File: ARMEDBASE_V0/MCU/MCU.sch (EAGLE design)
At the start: 35 parts, among them IC1 REG1117, IC2 MEGA8-P, K1 CQ1-12V, Q1 20Mhz, Q2 2N3904, Q3 2N3904

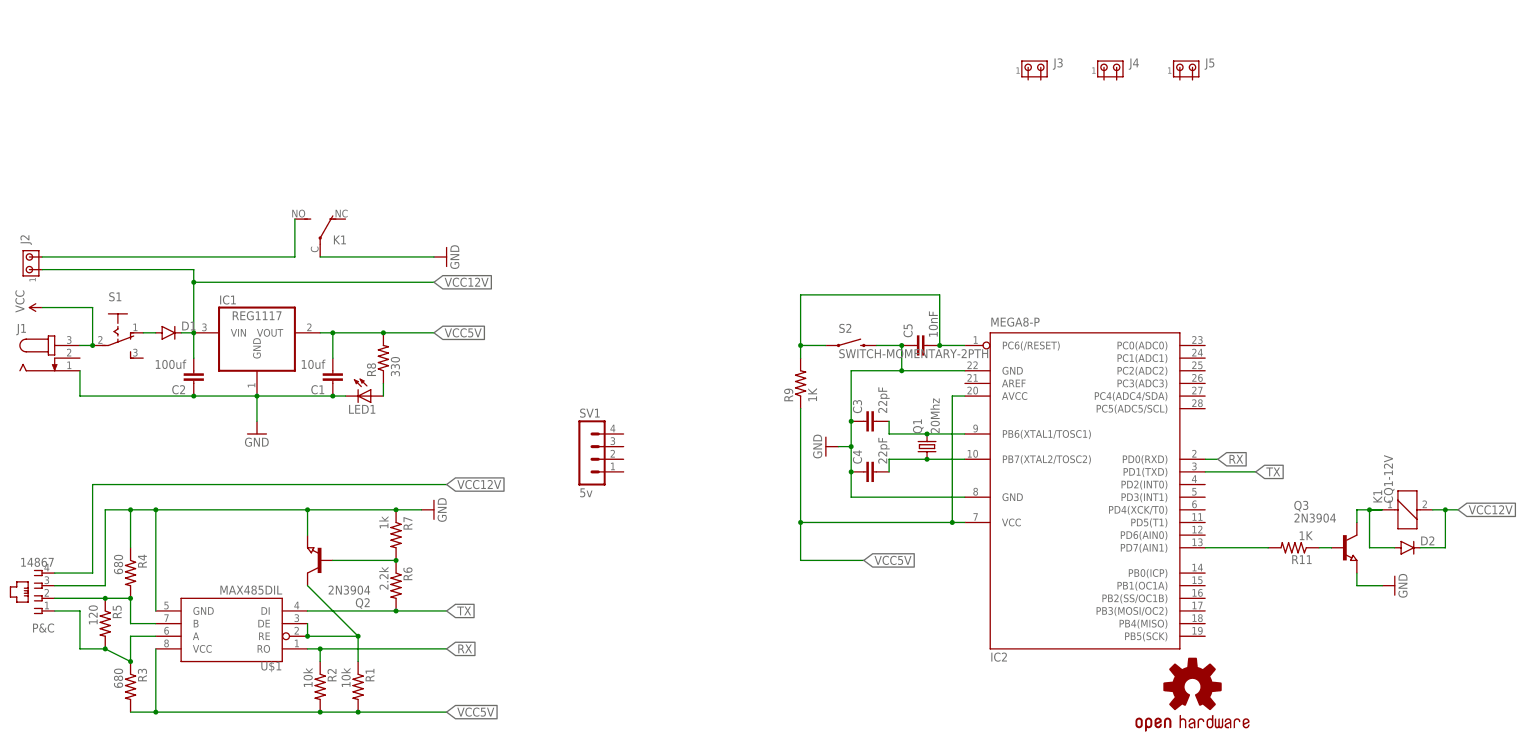
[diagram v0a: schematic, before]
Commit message: 7805
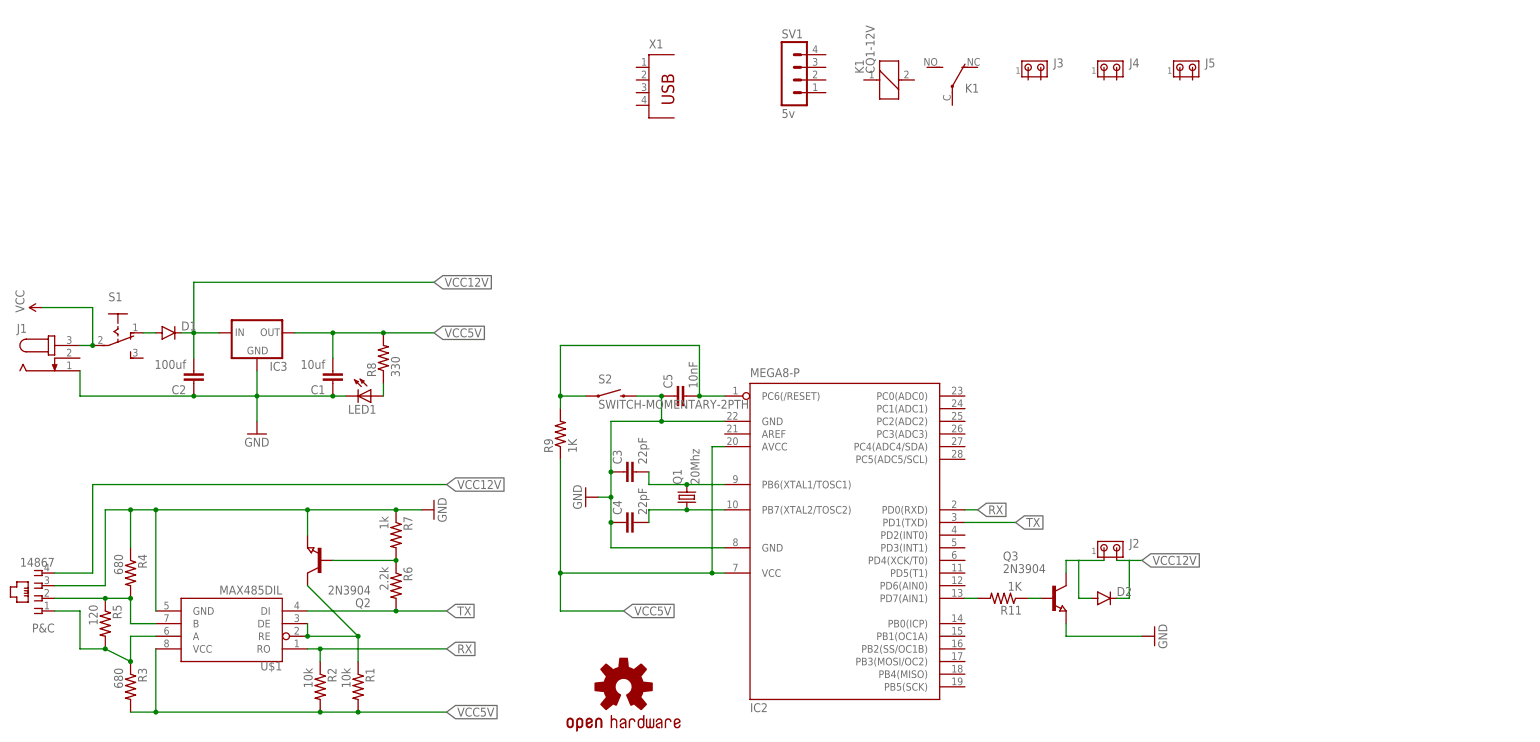
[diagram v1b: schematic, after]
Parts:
- removed IC1: REG1117, burr-brown:REG1117
- added IC3: (no value), SparkFun-PowerIC:V_REG_78XX-TO-220
- added X1: (no value), con-berg:PN87520
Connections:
- removed net N$1: J2.2, K12.S
- net GND: now also IC3.GND; no longer IC1.GND, K12.P
- net N$5: now also J2.1; no longer K11.1
- net VCC12V: now also IC3.IN, J2.2; no longer IC1.VIN, J2.1, K11.2
- net VCC5V: now also IC3.OUT; no longer IC1.VOUT
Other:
- moved on the sheet: C3, C4, C5, D2, IC2, J2, K1, Q1, Q3, R11, R9, S2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
